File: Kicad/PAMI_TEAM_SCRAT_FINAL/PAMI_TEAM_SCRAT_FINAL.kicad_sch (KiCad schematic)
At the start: 48 parts, among them J1 ALIM, J2 TOF, J3 IR, J4 M1, J5 M2, J6 XL320, SW1 BTN1, SW2 BTN2, SW3 BTN3, U3 WE-DC-DC-5V, U4 AZ1117CH2-3.3, U5 TB6612FNG, Y1 Crystal

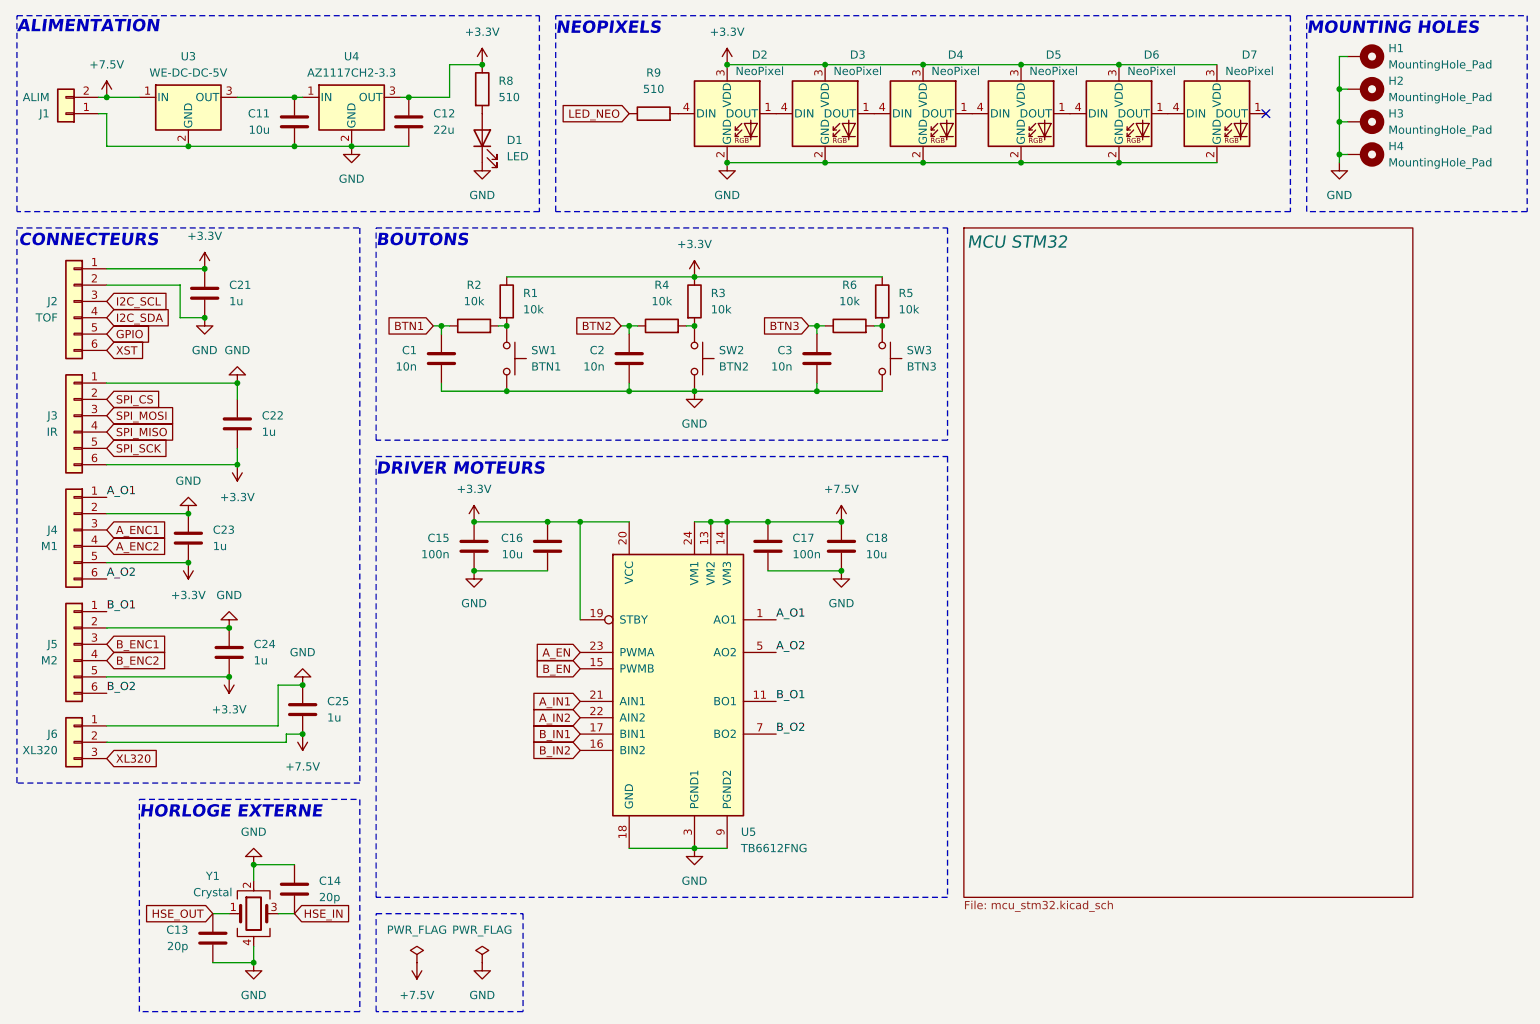
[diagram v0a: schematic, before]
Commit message: update pcb
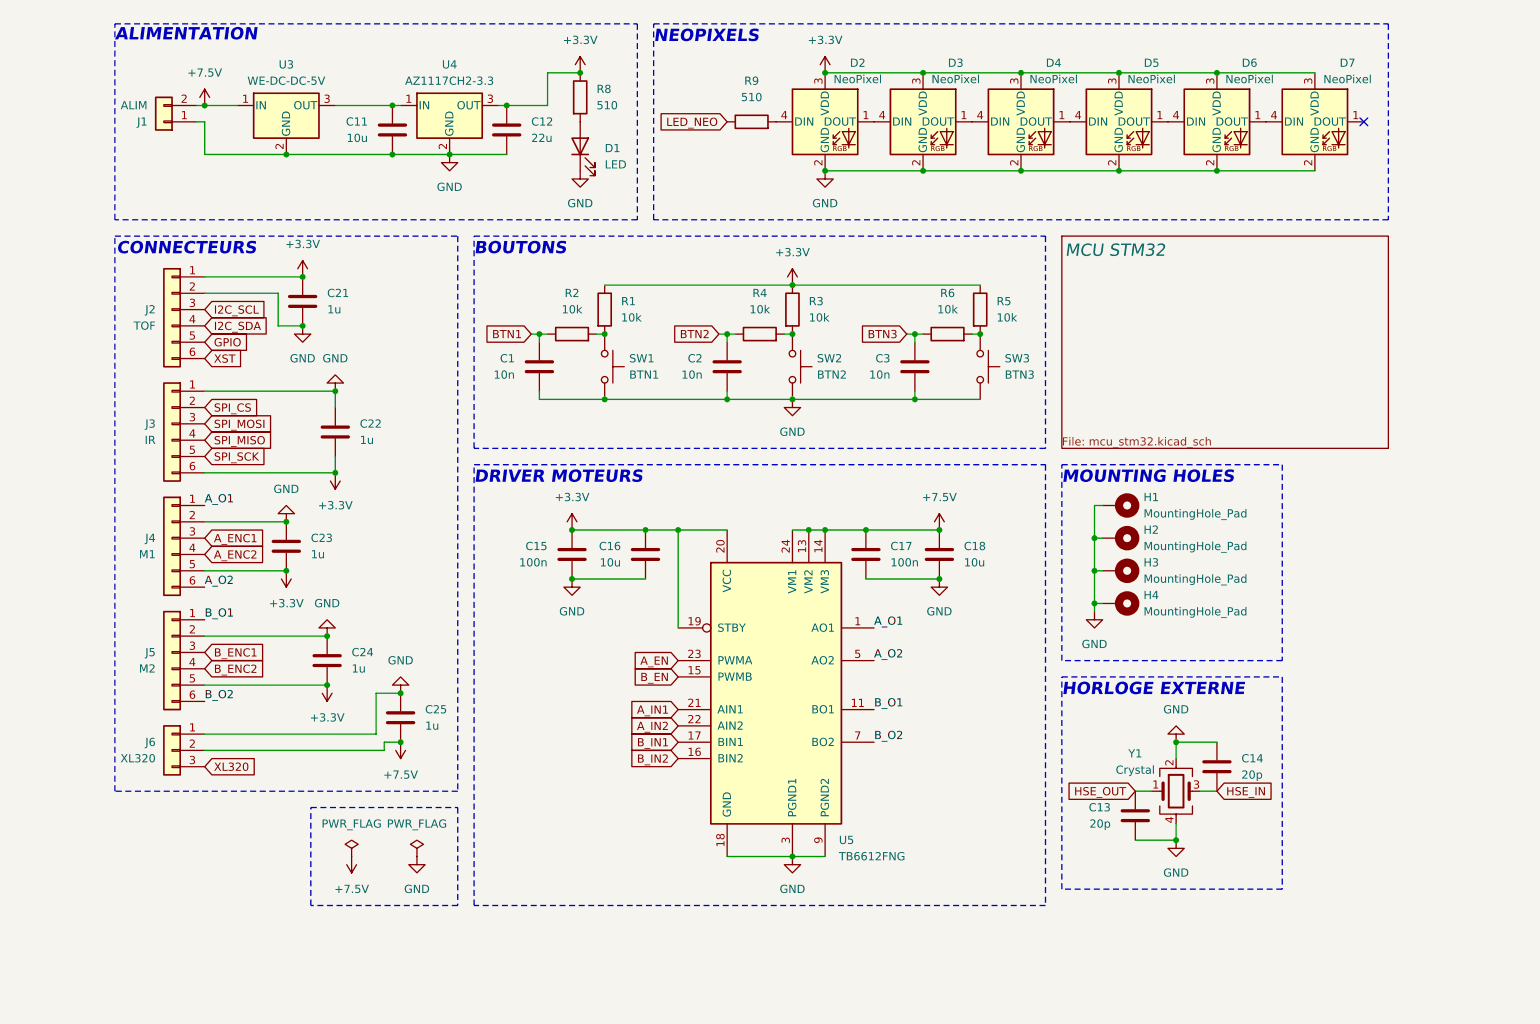
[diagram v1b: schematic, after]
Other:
- moved on the sheet: C1, C11, C12, C13, C14, C15, C16, C17, C18, C2, C21, C22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
